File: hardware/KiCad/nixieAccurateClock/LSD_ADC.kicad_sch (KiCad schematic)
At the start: 18 parts, among them U6 ADC0820BCWMX

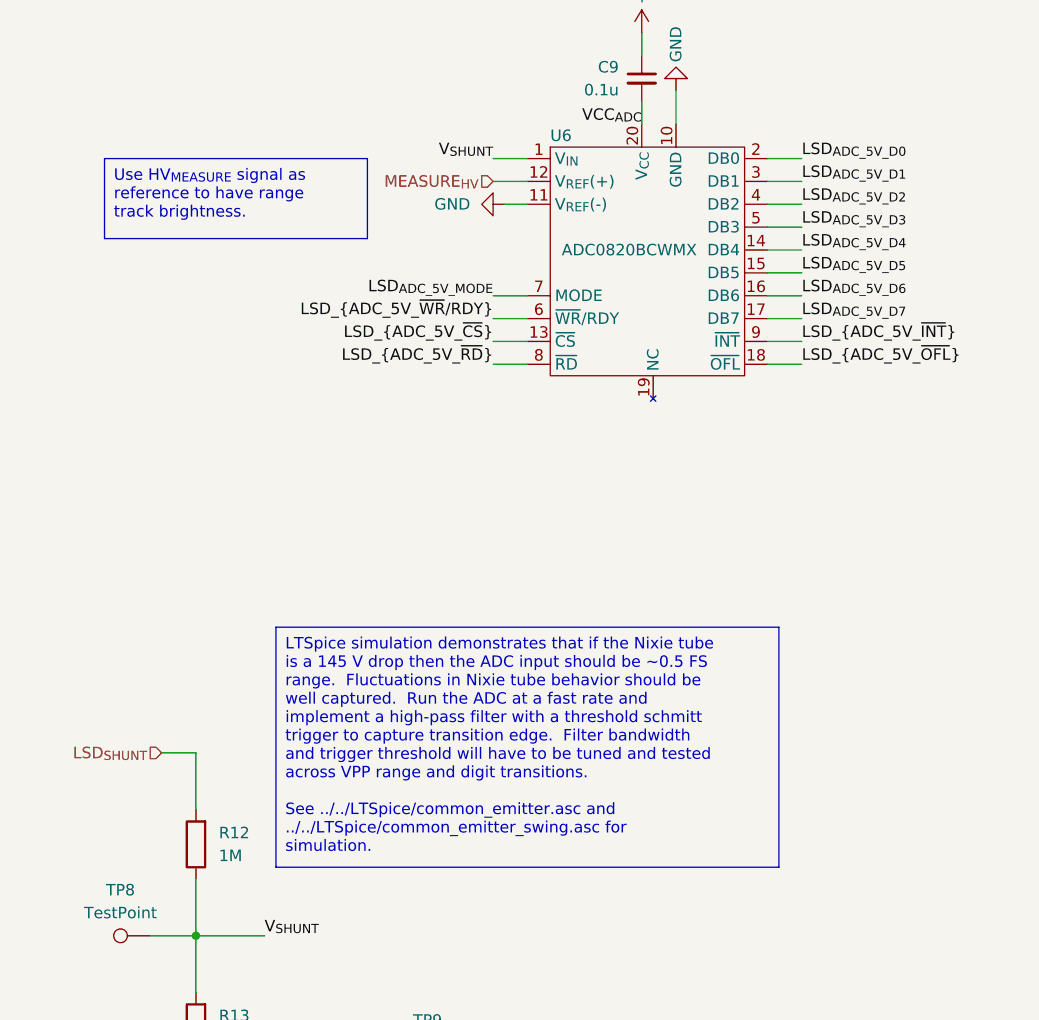
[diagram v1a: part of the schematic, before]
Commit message: Modify HV supply to attempt to solve weak IC
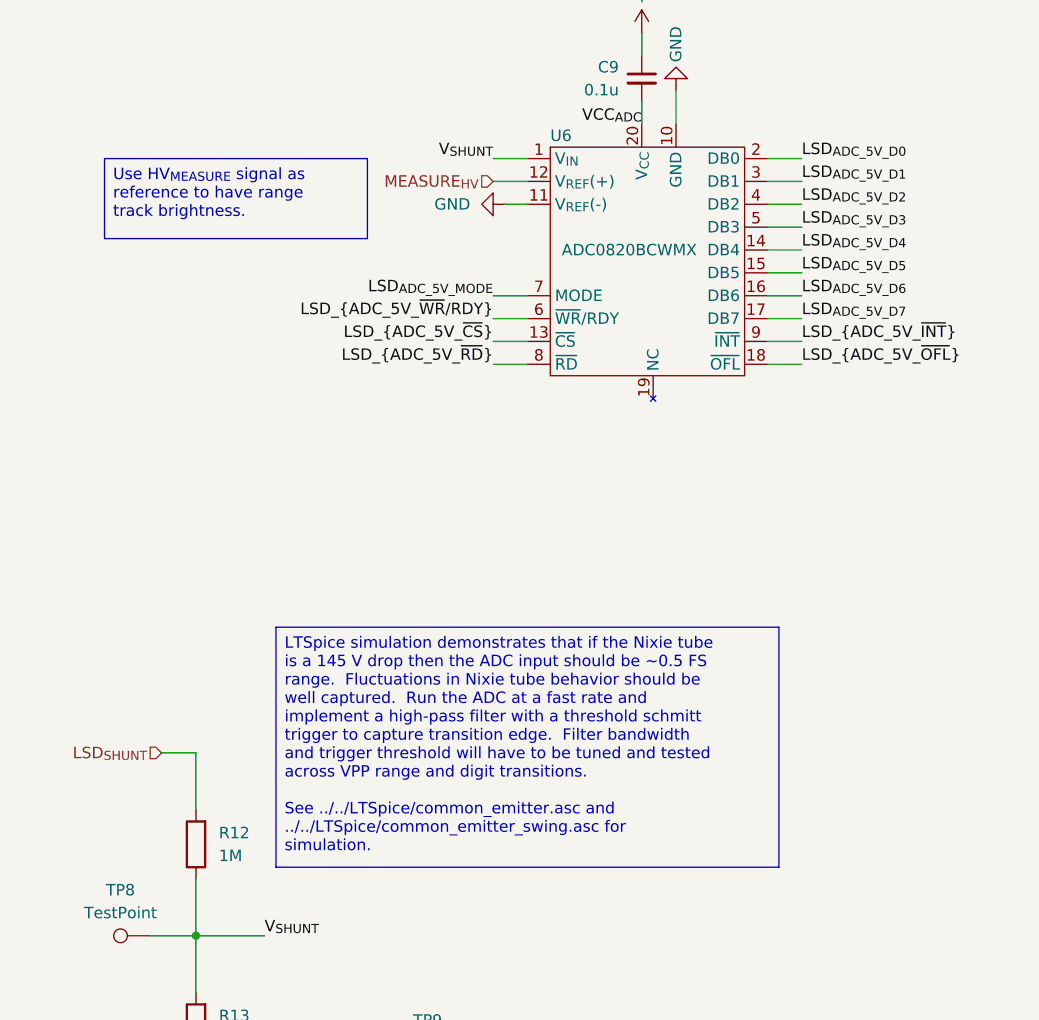
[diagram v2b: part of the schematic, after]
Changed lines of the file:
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@@
 (kicad_sch
-	(version 20231120)
+	(version 20250114)
 	(generator "eeschema")
-	(generator_version "8.0")
+	(generator_version "9.0")
 	(paper "A4")
 	(title_block
@@
 		(company "Paul Willis")
 	)
+	(text_box "Use HV_{MEASURE} signal as reference to have range track brightness."
+		(exclude_from_sim no)
+		(at 24.13 38.1 0)
+		(size 29.21 8.89)
+		(margins 0.9525 0.9525 0.9525 0.9525)
+		(stroke
+			(width 0)
+			(type default)
+		)
+		(fill
+			(type none)
+		)
+		(effects
+			(font
+				(size 1.27 1.27)
+			)
+			(justify left top)
+		)
+	)
+	(text_box "LTSpice simulation demonstrates that if the Nixie tube is a 145 V drop then the ADC input should be ~0.5 FS range.  Fluctuations in Nixie tube behavior should be well captured.  Run the ADC at a fast rate and implement a high-pass filter with a threshold schmitt trigger to capture transition edge.  Filter bandwidth and trigger threshold will have to be tuned and tested across VPP range and digit transitions.\n\nSee ../../LTSpice/common_emitter.asc and ../../LTSpice/common_emitter_swing.asc for simulation."
+		(exclude_from_sim no)
+		(at 43.18 90.17 0)
+		(size 55.88 26.67)
+		(margins 0.9525 0.9525 0.9525 0.9525)
+		(stroke
+			(width 0)
+			(type default)
+		)
+		(fill
+			(type none)
+		)
+		(effects
+			(font
+				(size 1.27 1.27)
+			)
+			(justify left top)
+		)
+	)
 	(junction
 		(at 157.48 105.41)
@@
 		)
 	)
-	(text_box "Use HV_{MEASURE} signal as reference to have range track brightness."
-		(exclude_from_sim no)
-		(at 24.13 38.1 0)
-		(size 29.21 8.89)
-		(stroke
-			(width 0)
-			(type default)
-		)
-		(fill
-			(type none)
-		)
-		(effects
-			(font
-				(size 1.27 1.27)
-			)
-			(justify left top)
-		)
-	)
-	(text_box "LTSpice simulation demonstrates that if the Nixie tube is a 145 V drop then the ADC input should be ~0.5 FS range.  Fluctuations in Nixie tube behavior should be well captured.  Run the ADC at a fast rate and implement a high-pass filter with a threshold schmitt trigger to capture transition edge.  Filter bandwidth and trigger threshold will have to be tuned and tested across VPP range and digit transitions.\n\nSee ../../LTSpice/common_emitter.asc and ../../LTSpice/common_emitter_swing.asc for simulation."
-		(exclude_from_sim no)
-		(at 43.18 90.17 0)
-		(size 55.88 26.67)
-		(stroke
-			(width 0)
-			(type default)
-		)
-		(fill
-			(type none)
-		)
-		(effects
-			(font
-				(size 1.27 1.27)
-			)
-			(justify left top)
-		)
-	)
 	(label "LSD_{ADC_5V_~{RD}}"
 		(at 247.65 113.03 0)
-		(fields_autoplaced yes)
 		(effects
 			(font
@@
 	(label "LSD_{ADC_5V_D6}"
 		(at 101.6 53.34 0)
-		(fields_autoplaced yes)
 		(effects
 			(font
@@
 	(label "LSD_{ADC_5V_D1}"
 		(at 156.21 53.34 180)
-		(fields_autoplaced yes)
 		(effects
 			(font
@@
 	(label "LSD_{ADC_5V_MODE}"
 		(at 67.31 53.34 180)
-		(fields_autoplaced yes)
 		(effects
 			(font
@@
 	(label "LSD_{ADC_5V_D2}"
 		(at 101.6 43.18 0)
-		(fields_autoplaced yes)
 		(effects
 			(font
@@
 	(label "LSD_{ADC_5V_~{OFL}}"
 		(at 101.6 60.96 0)
-		(fields_autoplaced yes)
 		(effects
 			(font
@@
 	(label "VCC_{lvl-shift-B-1}"
 		(at 189.23 41.91 180)
-		(fields_autoplaced yes)
 		(effects
 			(font
@@
 	(label "LSD_{ADC_5V_D2}"
 		(at 156.21 50.8 180)
-		(fields_autoplaced yes)
 		(effects
 			(font
@@
 	(label "VCC_{lvl-shift-B-2}"
 		(at 251.46 43.18 180)
-		(fields_autoplaced yes)
 		(effects
 			(font
@@
 	(label "LSD_{ADC_5V_~{CS}}"
 		(at 247.65 115.57 0)
-		(fields_autoplaced yes)
 		(effects
 			(font
@@
 	(label "LSD_{ADC_5V_D5}"
 		(at 101.6 50.8 0)
-		(fields_autoplaced yes)
 		(effects
 			(font
@@
 	(label "LSD_{ADC_5V_D0}"
 		(at 156.21 55.88 180)
-		(fields_autoplaced yes)
 		(effects
 			(font
@@
 	(label "LSD_{ADC_5V_D0}"
 		(at 101.6 38.1 0)
-		(fields_autoplaced yes)
 		(effects
 			(font
@@
 	(label "V_{SHUNT}"
 		(at 41.91 124.46 0)
-		(fields_autoplaced yes)
 		(effects
 			(font
@@
 	(label "VCC_{lvl-shift-A-3}"
 		(at 151.13 101.6 0)
-		(fields_autoplaced yes)
 		(effects
 			(font
@@
 	(label "VCC_{lvl-shift-B-4}"
 		(at 252.73 101.6 180)
-		(fields_autoplaced yes)
 		(effects
 			(font
@@
 	(label "LSD_{ADC_5V_D6}"
 		(at 218.44 52.07 180)
-		(fields_autoplaced yes)
 		(effects
 			(font
@@
 	(label "VCC_{lvl-shift-A-4}"
 		(at 214.63 101.6 0)
-		(fields_autoplaced yes)
 		(effects
 			(font
@@
 	(label "LSD_{ADC_5V_D3}"
 		(at 156.21 48.26 180)
-		(fields_autoplaced yes)
 		(effects
 			(font
@@
 	(label "LSD_{ADC_5V_D7}"
 		(at 101.6 55.88 0)
-		(fields_autoplaced yes)
 		(effects
 			(font
@@
 	(label "LSD_{ADC_5V_D4}"
 		(at 101.6 48.26 0)
-		(fields_autoplaced yes)
 		(effects
 			(font
@@
 	(label "LSD_{ADC_5V_~{WR}{slash}RDY}"
 		(at 67.31 55.88 180)
-		(fields_autoplaced yes)
 		(effects
 			(font
@@
 	(label "LSD_{ADC_5V_~{CS}}"
 		(at 67.31 58.42 180)
-		(fields_autoplaced yes)
 		(effects
 			(font
@@
 	(label "LSD_{ADC_5V_D5}"
 		(at 218.44 54.61 180)
-		(fields_autoplaced yes)
 		(effects
 			(font
@@
 	(label "VCC_{lvl-shift-B-3}"
 		(at 189.23 101.6 180)
-		(fields_autoplaced yes)
 		(effects
 			(font
@@
 	(label "LSD_{ADC_5V_D4}"
 		(at 218.44 57.15 180)
-		(fields_autoplaced yes)
 		(effects
 			(font
@@
 	(label "VCC_{lvl-shift-A-2}"
 		(at 213.36 43.18 0)
-		(fields_autoplaced yes)
 		(effects
 			(font
@@
 	(label "LSD_{ADC_5V_MODE}"
 		(at 247.65 110.49 0)
-		(fields_autoplaced yes)
 		(effects
 			(font
@@
 	(label "VCC_{lvl-shift-A-1}"
 		(at 151.13 41.91 0)
-		(fields_autoplaced yes)
 		(effects
 			(font
@@
 	(label "LSD_{ADC_5V_~{INT}}"
 		(at 156.21 115.57 180)
-		(fields_autoplaced yes)
 		(effects
 			(font
@@
 	(label "LSD_{ADC_5V_~{RD}}"
 		(at 67.31 60.96 180)
-		(fields_autoplaced yes)
 		(effects
 			(font
@@
 	(label "LSD_{ADC_5V_D1}"
 		(at 101.6 40.64 0)
-		(fields_autoplaced yes)
 		(effects
 			(font
@@
 	(label "V_{SHUNT}"
 		(at 67.31 38.1 180)
-		(fields_autoplaced yes)
 		(effects
 			(font
@@
 	(label "LSD_{ADC_5V_~{WR}{slash}RDY}"
 		(at 247.65 107.95 0)
-		(fields_autoplaced yes)
 		(effects
 			(font
@@
 	(label "LSD_{ADC_5V_~{INT}}"
 		(at 101.6 58.42 0)
-		(fields_autoplaced yes)
 		(effects
 			(font
@@
 	(label "LSD_{ADC_5V_~{OFL}}"
 		(at 156.21 113.03 180)
-		(fields_autoplaced yes)
 		(effects
 			(font
@@
 	(label "LSD_{ADC_5V_D7}"
 		(at 218.44 49.53 180)
-		(fields_autoplaced yes)
 		(effects
 			(font
@@
 	(label "LSD_{ADC_5V_D3}"
 		(at 101.6 45.72 0)
-		(fields_autoplaced yes)
 		(effects
 			(font
@@
 	(label "VCC_{ADC}"
 		(at 83.82 34.29 180)
-		(fields_autoplaced yes)
 		(effects
 			(font
@@
 		(shape output)
 		(at 184.15 113.03 0)
-		(fields_autoplaced yes)
 		(effects
 			(font
@@
 		(shape input)
 		(at 67.31 40.64 180)
-		(fields_autoplaced yes)
 		(effects
 			(font
@@
 		(shape output)
 		(at 246.38 52.07 0)
-		(fields_autoplaced yes)
 		(effects
 			(font
@@
 		(shape input)
 		(at 219.71 115.57 180)
-		(fields_autoplaced yes)
 		(effects
 			(font
@@
 		(shape output)
 		(at 184.15 53.34 0)
-		(fields_autoplaced yes)
 		(effects
 			(font
@@
 		(shape input)
 		(at 219.71 113.03 180)
-		(fields_autoplaced yes)
 		(effects
 			(font
@@
 		(shape output)
 		(at 184.15 50.8 0)
-		(fields_autoplaced yes)
 		(effects
 			(font
@@
 		(shape output)
 		(at 246.38 54.61 0)
-		(fields_autoplaced yes)
 		(effects
 			(font
@@
 		(shape input)
 		(at 219.71 107.95 180)
-		(fields_autoplaced yes)
 		(effects
 			(font
@@
 		(shape input)
 		(at 219.71 110.49 180)
-		(fields_autoplaced yes)
 		(effects
 			(font
@@
 		(shape input)
 		(at 30.48 104.14 180)
-		(fields_autoplaced yes)
 		(effects
 			(font
@@
 		(shape output)
 		(at 246.38 49.53 0)
-		(fields_autoplaced yes)
 		(effects
 			(font
@@
 		(shape output)
 		(at 246.38 57.15 0)
-		(fields_autoplaced yes)
 		(effects
 			(font
@@
 		(shape output)
 		(at 184.15 48.26 0)
-		(fields_autoplaced yes)
 		(effects
 			(font
@@
 		(shape output)
 		(at 184.15 115.57 0)
-		(fields_autoplaced yes)
 		(effects
 			(font
@@
 		(shape output)
 		(at 184.15 55.88 0)
-		(fields_autoplaced yes)
-		(effects
-			(font
+		(effects
+			(font
